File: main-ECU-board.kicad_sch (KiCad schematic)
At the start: 13 parts, among them IC1 R7FA4M1AB3CFM#AA0, J1 Power, J2 Analog, J3 Digital/PWM, J4 Digital/PWM, J5 USB_C_Receptacle, J6 Conn_01x02_Pin

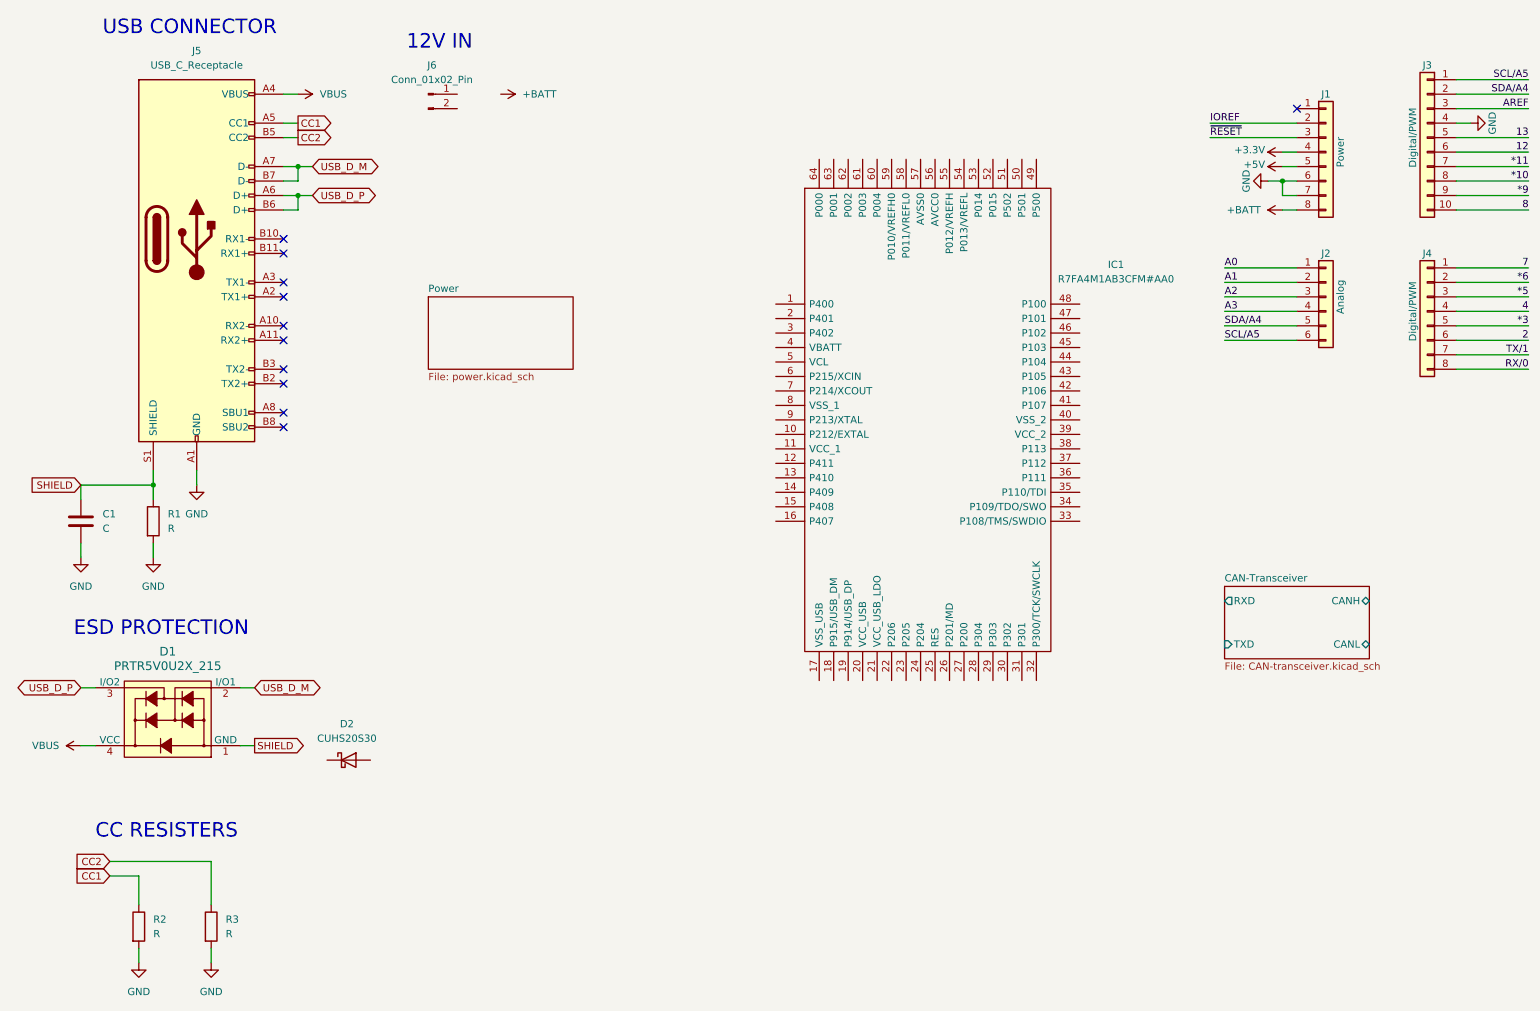
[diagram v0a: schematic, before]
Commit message: almost completed power, can, mcu
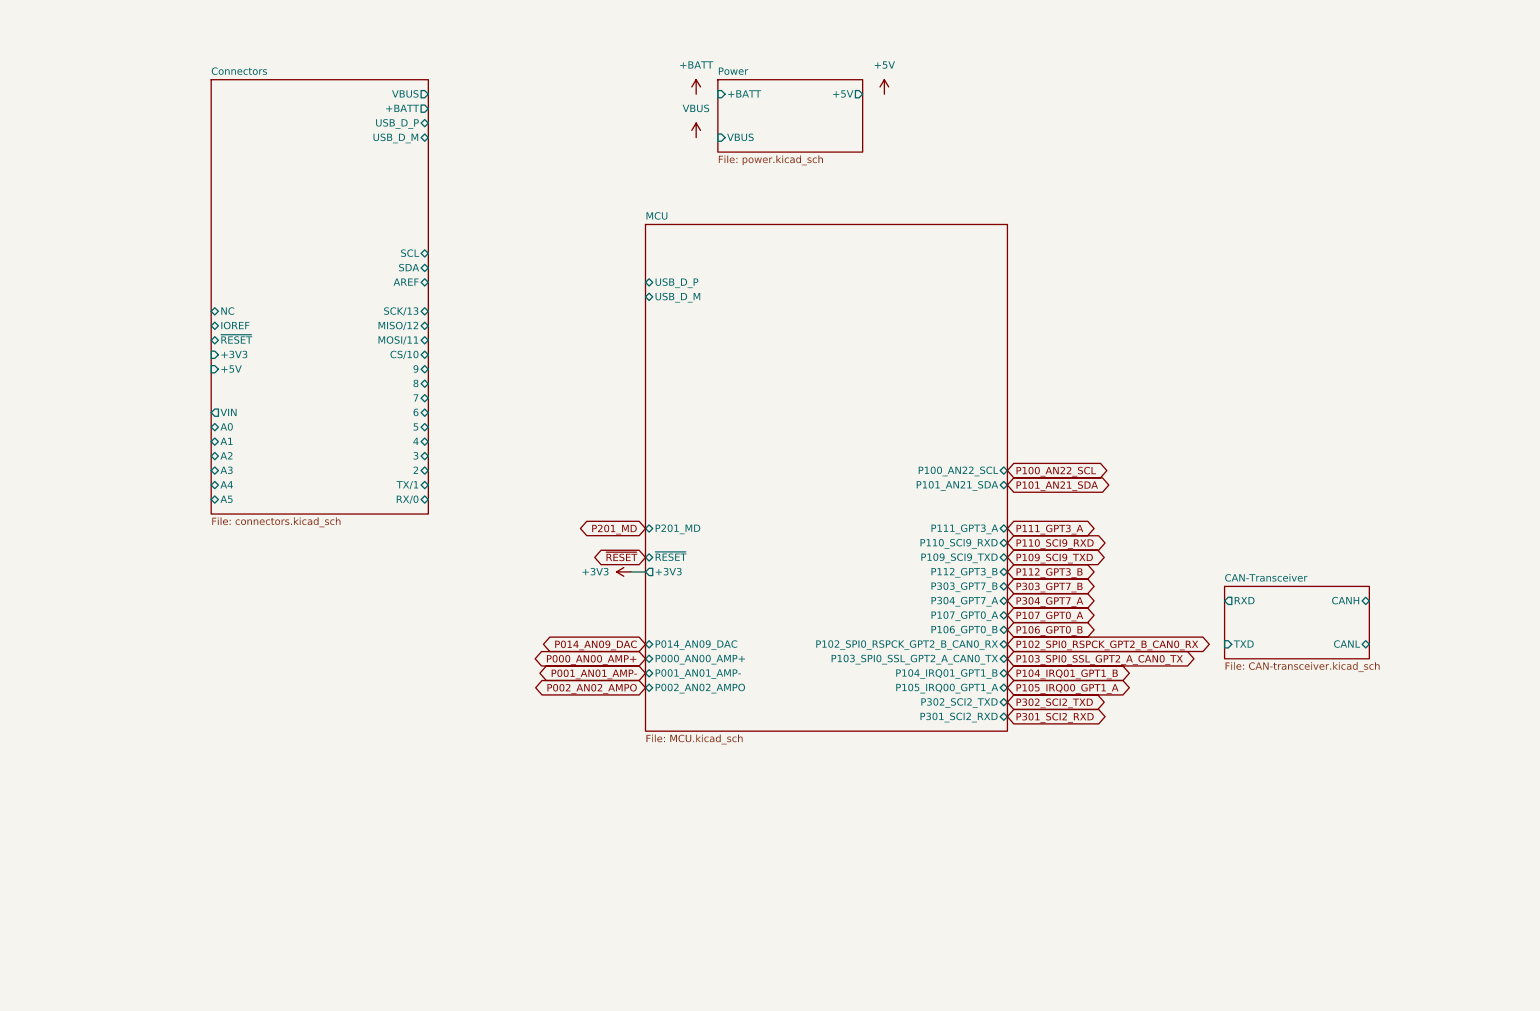
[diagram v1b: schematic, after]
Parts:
- removed C1: C, symbol Device:C
- removed D1: PRTR5V0U2X_215, digikey-footprints:TO-253-4, symbol dk_TVS-Diodes:PRTR5V0U2X_215
- removed D2: CUHS20S30, SamacSys_Parts:CUHS20S40H3F, symbol Device:D_Schottky
- removed IC1: R7FA4M1AB3CFM#AA0, QFP50P1200X1200X170-64N, symbol SamacSys_Parts:R7FA4M1AB3CFM#AA0
- removed J1: Power, Connector_PinSocket_2.54mm:PinSocket_1x08_P2.54mm_Vertical, symbol Connector_Generic:Conn_01x08
- removed J2: Analog, Connector_PinSocket_2.54mm:PinSocket_1x06_P2.54mm_Vertical, symbol Connector_Generic:Conn_01x06
- removed J3: Digital/PWM, Connector_PinSocket_2.54mm:PinSocket_1x10_P2.54mm_Vertical, symbol Connector_Generic:Conn_01x10
- removed J4: Digital/PWM, Connector_PinSocket_2.54mm:PinSocket_1x08_P2.54mm_Vertical, symbol Connector_Generic:Conn_01x08
- removed J5: USB_C_Receptacle, SamacSys_Parts:5077CR-16-SMC2-BK-TR, symbol Connector:USB_C_Receptacle
- removed J6: Conn_01x02_Pin, symbol Connector:Conn_01x02_Pin
- removed R1, R2, R3: R, symbol Device:R
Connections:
- no-connect marks 11 -> 0
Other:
- added sheet Connectors (connectors.kicad_sch)
- added sheet MCU (MCU.kicad_sch)
- sheet Power ports: added +5V, +BATT, VBUS; removed none
- note removed: "12V IN"
- note removed: "CC RESISTERS"
- note removed: "ESD PROTECTION"
- note removed: "USB CONNECTOR"

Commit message: add, modify
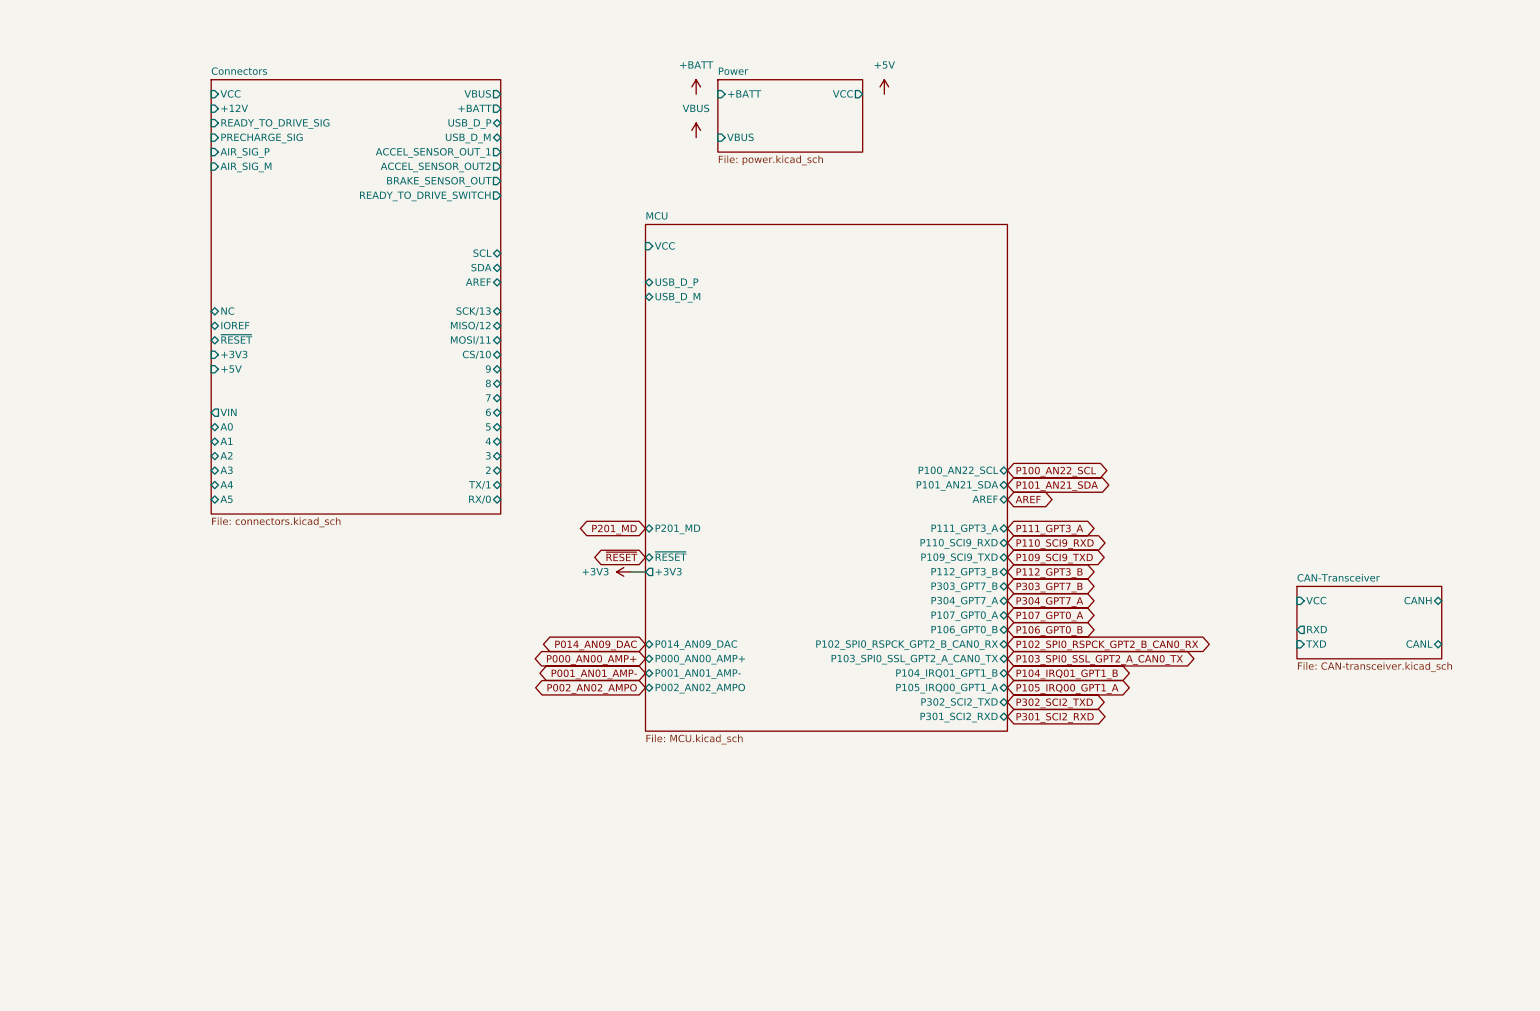
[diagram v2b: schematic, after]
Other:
- sheet CAN-Transceiver ports: added VCC; removed none
- sheet Connectors ports: added +12V, ACCEL_SENSOR_OUT2, ACCEL_SENSOR_OUT_1, AIR_SIG_M, AIR_SIG_P, BRAKE_SENSOR_OUT, PRECHARGE_SIG, READY_TO_DRIVE_SIG, READY_TO_DRIVE_SWITCH, VCC; removed none
- sheet MCU ports: added AREF, VCC; removed none
- sheet Power ports: added VCC; removed +5V
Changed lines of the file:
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@@
+    )
+  )
+  (global_label "AREF" (shape bidirectional) (at 190.5 99.06 0) (fields_autoplaced)
+    (effects (font (size 1.27 1.27)) (justify left))
+    (property "Intersheetrefs" "${INTERSHEET_REFS}" (at 199.1927 99.06 0)
+      (effects (font (size 1.27 1.27)) (justify left) hide)
     )
   )
@@
     )
   )
-  (sheet (at 50.8 25.4) (size 38.1 76.2) (fields_autoplaced)
+  (sheet (at 50.8 25.4) (size 50.8 76.2) (fields_autoplaced)
     (stroke (width 0.1524) (type solid))
     (fill (color 0 0 0 0.0000))
@@
       (effects (font (size 1.27 1.27)) (justify left top))
     )
-    (pin "VBUS" output (at 88.9 27.94 0)
-      (effects (font (size 1.27 1.27)) (justify right))
-    )
-    (pin "+BATT" output (at 88.9 30.48 0)
-      (effects (font (size 1.27 1.27)) (justify right))
-    )
-    (pin "USB_D_M" bidirectional (at 88.9 35.56 0)
-      (effects (font (size 1.27 1.27)) (justify right))
-    )
-    (pin "USB_D_P" bidirectional (at 88.9 33.02 0)
-      (effects (font (size 1.27 1.27)) (justify right))
-    )
-    (pin "2" bidirectional (at 88.9 93.98 0)
-      (effects (font (size 1.27 1.27)) (justify right))
-    )
-    (pin "TX{slash}1" bidirectional (at 88.9 96.52 0)
-      (effects (font (size 1.27 1.27)) (justify right))
-    )
-    (pin "RX{slash}0" bidirectional (at 88.9 99.06 0)
-      (effects (font (size 1.27 1.27)) (justify right))
-    )
-    (pin "SCL" bidirectional (at 88.9 55.88 0)
-      (effects (font (size 1.27 1.27)) (justify right))
-    )
-    (pin "SDA" bidirectional (at 88.9 58.42 0)
-      (effects (font (size 1.27 1.27)) (justify right))
-    )
-    (pin "CS{slash}10" bidirectional (at 88.9 73.66 0)
-      (effects (font (size 1.27 1.27)) (justify right))
-    )
-    (pin "MOSI{slash}11" bidirectional (at 88.9 71.12 0)
-      (effects (font (size 1.27 1.27)) (justify right))
-    )
-    (pin "MISO{slash}12" bidirectional (at 88.9 68.58 0)
-      (effects (font (size 1.27 1.27)) (justify right))
-    )
-    (pin "SCK{slash}13" bidirectional (at 88.9 66.04 0)
-      (effects (font (size 1.27 1.27)) (justify right))
-    )
-    (pin "9" bidirectional (at 88.9 76.2 0)
-      (effects (font (size 1.27 1.27)) (justify right))
-    )
-    (pin "8" bidirectional (at 88.9 78.74 0)
-      (effects (font (size 1.27 1.27)) (justify right))
-    )
-    (pin "3" bidirectional (at 88.9 91.44 0)
-      (effects (font (size 1.27 1.27)) (justify right))
-    )
-    (pin "5" bidirectional (at 88.9 86.36 0)
-      (effects (font (size 1.27 1.27)) (justify right))
-    )
-    (pin "4" bidirectional (at 88.9 88.9 0)
-      (effects (font (size 1.27 1.27)) (justify right))
-    )
-    (pin "6" bidirectional (at 88.9 83.82 0)
-      (effects (font (size 1.27 1.27)) (justify right))
-    )
-    (pin "7" bidirectional (at 88.9 81.28 0)
-      (effects (font (size 1.27 1.27)) (justify right))
-    )
-    (pin "AREF" bidirectional (at 88.9 60.96 0)
+    (pin "VBUS" output (at 101.6 27.94 0)
+      (effects (font (size 1.27 1.27)) (justify right))
+    )
+    (pin "+BATT" output (at 101.6 30.48 0)
+      (effects (font (size 1.27 1.27)) (justify right))
+    )
+    (pin "USB_D_M" bidirectional (at 101.6 35.56 0)
+      (effects (font (size 1.27 1.27)) (justify right))
+    )
+    (pin "USB_D_P" bidirectional (at 101.6 33.02 0)
+      (effects (font (size 1.27 1.27)) (justify right))
+    )
+    (pin "2" bidirectional (at 101.6 93.98 0)
+      (effects (font (size 1.27 1.27)) (justify right))
+    )
+    (pin "TX{slash}1" bidirectional (at 101.6 96.52 0)
+      (effects (font (size 1.27 1.27)) (justify right))
+    )
+    (pin "RX{slash}0" bidirectional (at 101.6 99.06 0)
+      (effects (font (size 1.27 1.27)) (justify right))
+    )
+    (pin "SCL" bidirectional (at 101.6 55.88 0)
+      (effects (font (size 1.27 1.27)) (justify right))
+    )
+    (pin "SDA" bidirectional (at 101.6 58.42 0)
+      (effects (font (size 1.27 1.27)) (justify right))
+    )
+    (pin "CS{slash}10" bidirectional (at 101.6 73.66 0)
+      (effects (font (size 1.27 1.27)) (justify right))
+    )
+    (pin "MOSI{slash}11" bidirectional (at 101.6 71.12 0)
+      (effects (font (size 1.27 1.27)) (justify right))
+    )
+    (pin "MISO{slash}12" bidirectional (at 101.6 68.58 0)
+      (effects (font (size 1.27 1.27)) (justify right))
+    )
+    (pin "SCK{slash}13" bidirectional (at 101.6 66.04 0)
+      (effects (font (size 1.27 1.27)) (justify right))
+    )
+    (pin "9" bidirectional (at 101.6 76.2 0)
+      (effects (font (size 1.27 1.27)) (justify right))
+    )
+    (pin "8" bidirectional (at 101.6 78.74 0)
+      (effects (font (size 1.27 1.27)) (justify right))
+    )
+    (pin "3" bidirectional (at 101.6 91.44 0)
+      (effects (font (size 1.27 1.27)) (justify right))
+    )
+    (pin "5" bidirectional (at 101.6 86.36 0)
+      (effects (font (size 1.27 1.27)) (justify right))
+    )
+    (pin "4" bidirectional (at 101.6 88.9 0)
+      (effects (font (size 1.27 1.27)) (justify right))
+    )
+    (pin "6" bidirectional (at 101.6 83.82 0)
+      (effects (font (size 1.27 1.27)) (justify right))
+    )
+    (pin "7" bidirectional (at 101.6 81.28 0)
+      (effects (font (size 1.27 1.27)) (justify right))
+    )
+    (pin "AREF" bidirectional (at 101.6 60.96 0)
       (effects (font (size 1.27 1.27)) (justify right))
     )
@@
     )
     (pin "A2" bidirectional (at 50.8 91.44 180)
+      (effects (font (size 1.27 1.27)) (justify left))
+    )
+    (pin "VCC" input (at 50.8 27.94 180)
+      (effects (font (size 1.27 1.27)) (justify left))
+    )
+    (pin "BRAKE_SENSOR_OUT" output (at 101.6 43.18 0)
+      (effects (font (size 1.27 1.27)) (justify right))
+    )
+    (pin "ACCEL_SENSOR_OUT_1" output (at 101.6 38.1 0)
+      (effects (font (size 1.27 1.27)) (justify right))
+    )
+    (pin "ACCEL_SENSOR_OUT2" output (at 101.6 40.64 0)
+      (effects (font (size 1.27 1.27)) (justify right))
+    )
+    (pin "READY_TO_DRIVE_SIG" input (at 50.8 33.02 180)
+      (effects (font (size 1.27 1.27)) (justify left))
+    )
+    (pin "+12V" input (at 50.8 30.48 180)
+      (effects (font (size 1.27 1.27)) (justify left))
+    )
+    (pin "READY_TO_DRIVE_SWITCH" output (at 101.6 45.72 0)
+      (effects (font (size 1.27 1.27)) (justify right))
+    )
+    (pin "AIR_SIG_M" input (at 50.8 40.64 180)
+      (effects (font (size 1.27 1.27)) (justify left))
+    )
+    (pin "AIR_SIG_P" input (at 50.8 38.1 180)
+      (effects (font (size 1.27 1.27)) (justify left))
+    )
+    (pin "PRECHARGE_SIG" input (at 50.8 35.56 180)
       (effects (font (size 1.27 1.27)) (justify left))
     )
@@
       (effects (font (size 1.27 1.27)) (justify left))
     )
-    (pin "+5V" output (at 165.1 27.94 0)
+    (pin "VCC" output (at 165.1 27.94 0)
       (effects (font (size 1.27 1.27)) (justify right))
     )
@@
     )
   )
-  (sheet (at 228.6 114.3) (size 25.4 12.7) (fields_autoplaced)
+  (sheet (at 241.3 114.3) (size 25.4 12.7) (fields_autoplaced)
     (stroke (width 0.1524) (type solid))
     (fill (color 0 0 0 0.0000))
-    (property "Sheetname" "CAN-Transceiver" (at 228.6 113.5884 0)
+    (property "Sheetname" "CAN-Transceiver" (at 241.3 113.5884 0)
       (effects (font (size 1.27 1.27)) (justify left bottom))
     )
-    (property "Sheetfile" "CAN-transceiver.kicad_sch" (at 228.6 127.5846 0)
+    (property "Sheetfile" "CAN-transceiver.kicad_sch" (at 241.3 127.5846 0)
       (effects (font (size 1.27 1.27)) (justify left top))
     )
-    (pin "RXD" output (at 228.6 116.84 180)
-      (effects (font (size 1.27 1.27)) (justify left))
-    )
-    (pin "TXD" input (at 228.6 124.46 180)
-      (effects (font (size 1.27 1.27)) (justify left))
-    )
-    (pin "CANH" bidirectional (at 254 116.84 0)
-      (effects (font (size 1.27 1.27)) (justify right))
-    )
-    (pin "CANL" bidirectional (at 254 124.46 0)
-      (effects (font (size 1.27 1.27)) (justify right))
+    (pin "RXD" output (at 241.3 121.92 180)
+      (effects (font (size 1.27 1.27)) (justify left))
+    )
+    (pin "TXD" input (at 241.3 124.46 180)
+      (effects (font (size 1.27 1.27)) (justify left))
+    )
+    (pin "CANH" bidirectional (at 266.7 116.84 0)
+      (effects (font (size 1.27 1.27)) (justify right))
+    )
+    (pin "CANL" bidirectional (at 266.7 124.46 0)
+      (effects (font (size 1.27 1.27)) (justify right))
+    )
+    (pin "VCC" input (at 241.3 116.84 180)
+      (effects (font (size 1.27 1.27)) (justify left))
     )
     (instances
@@
       (effects (font (size 1.27 1.27)) (justify left))
     )
-    (instances
+    (pin "VCC" input (at 127 54.61 180)
+      (effects (font (size 1.27 1.27)) (justify left))
+    )
+    (pin "AREF" bidirectional (at 190.5 99.06 0)
+      (effects (font (size 1.27 1.27)) (justify right))
+    )
+    (instances
